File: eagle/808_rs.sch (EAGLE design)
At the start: 75 parts, among them IC1 TL072P, IC2 TL072P, Q59 2N3904, Q60 2N3906, Q61 2N3904, Q62 2N3904, Q63 2N3904, Q74 MPF102, SW8 808_LT_MSS42_SW_4PDT

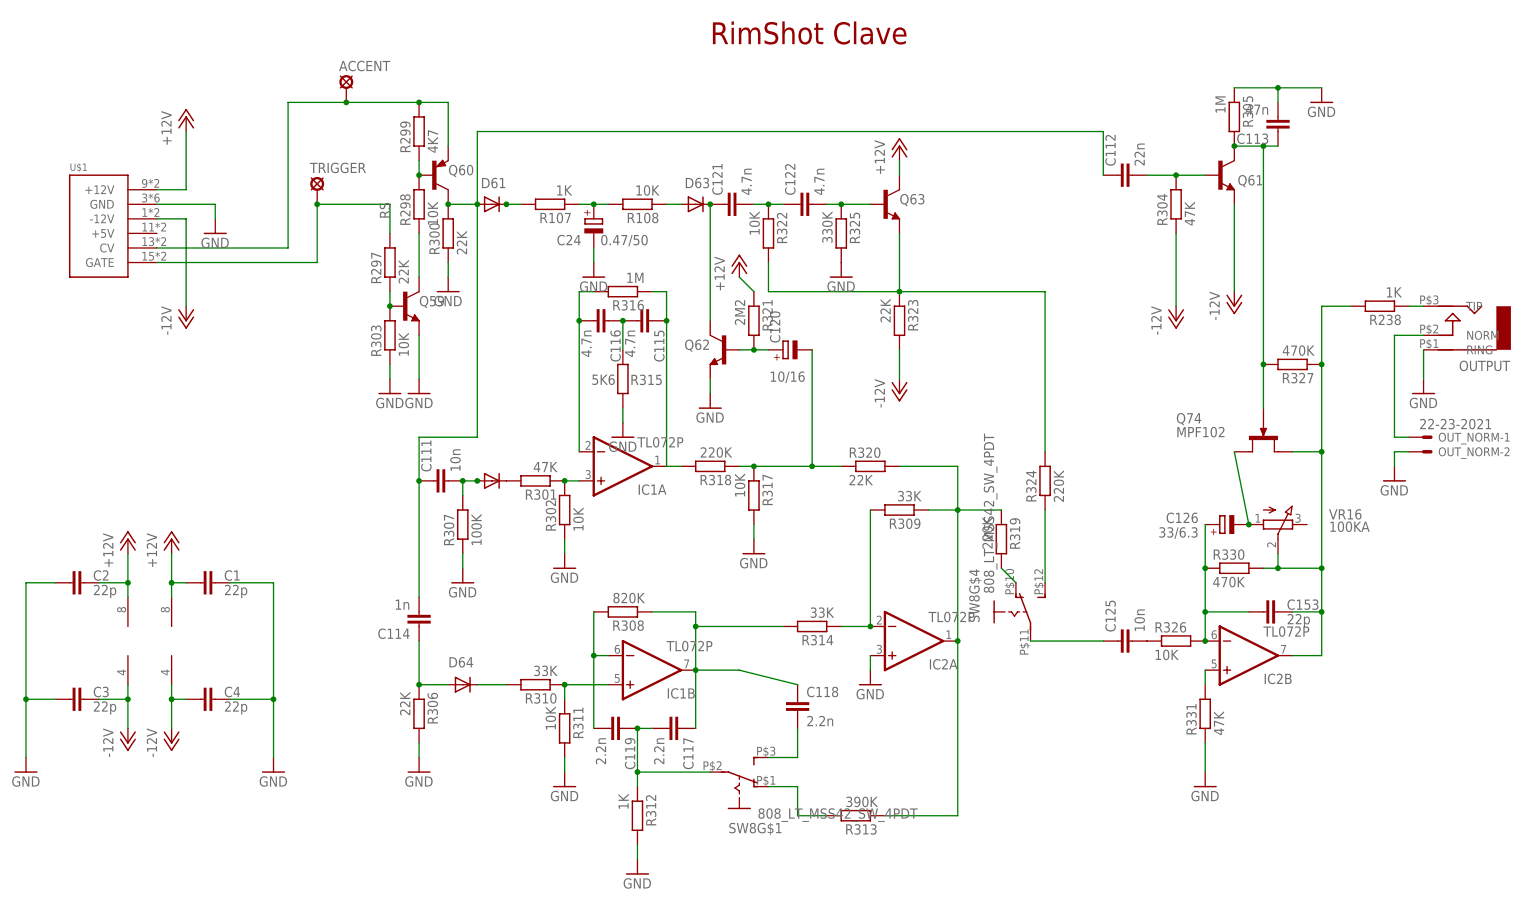
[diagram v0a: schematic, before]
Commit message: 2sk30
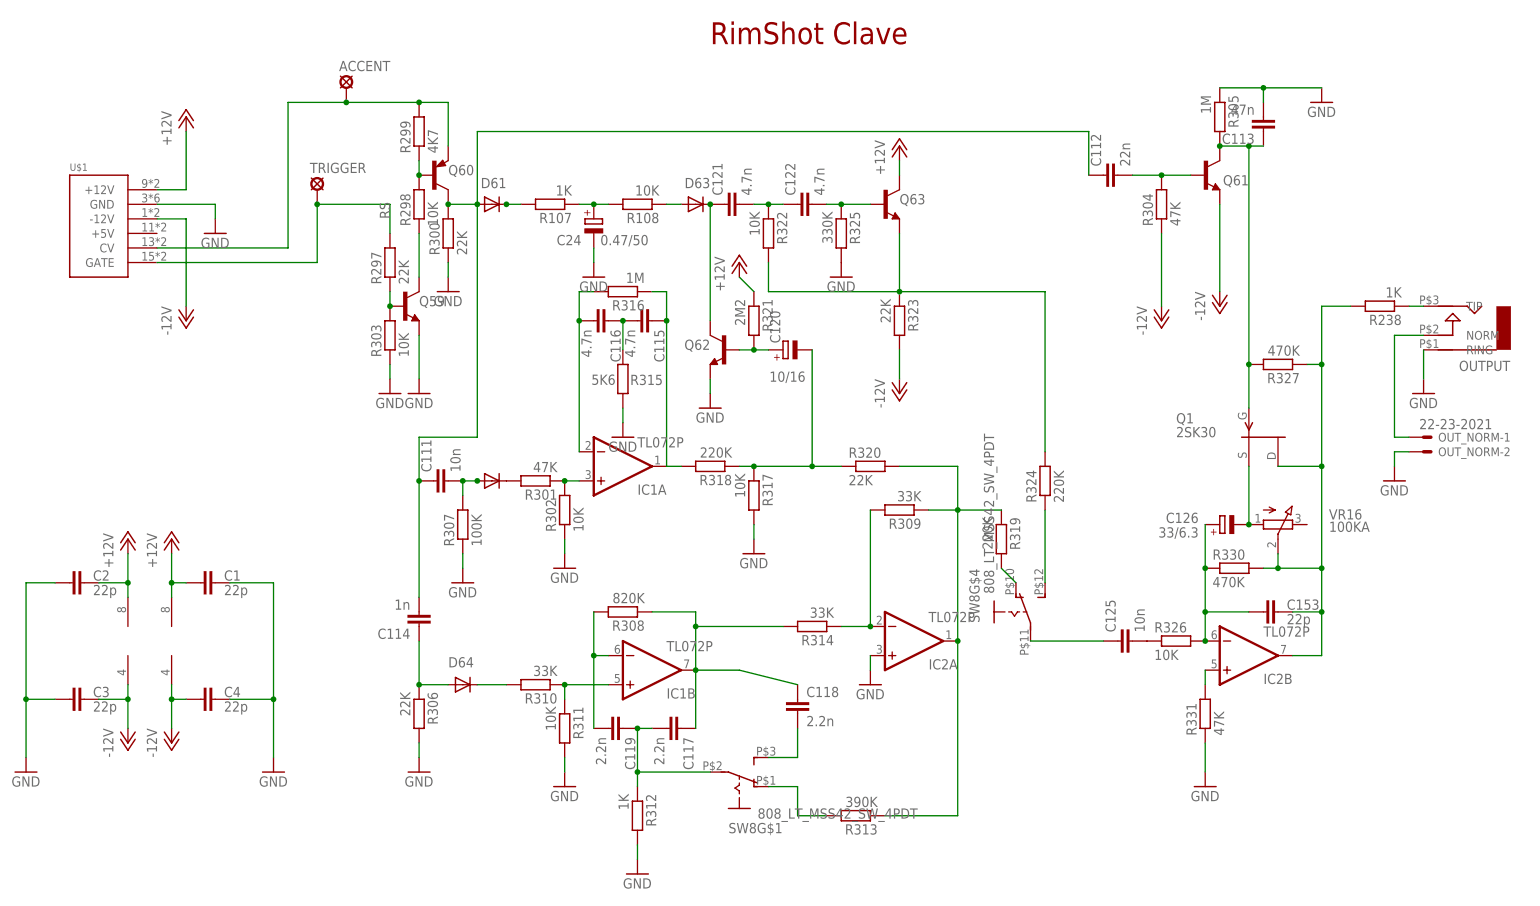
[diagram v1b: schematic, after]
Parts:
- removed Q74: MPF102, mes_transistors:MPF102
- added Q1: 2SK30, 808:2SK30
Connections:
- removed net N$170: C153.2, IC2B.OUT, Q74.D, R238.2, R327.1, R330.2, VR16.S
- new net N$8: C153.2, IC2B.OUT, Q1.D, R238.2, R327.1, R330.2, VR16.S
- net N$161: now also Q1.G; no longer Q74.G
- net N$351: now also Q1.S; no longer Q74.S
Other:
- moved on the sheet: C112, C113, Q61, R304, R305, R327
